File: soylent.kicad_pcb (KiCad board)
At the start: 2 copper layers, 33 x 42.2 mm, 31 parts, among them J1 DB9_Female, J2 Conn_01x04, J3 Conn_01x04, J4 Conn_02x03_Counter_Clockwise, Q1 BC847, Q2 BC847, U1 ATtiny202-SS, U2 MIC5504-3.3YM5, U3 LM2776, U4 MAX3188EEUT+T, U5 TLV6001DCK

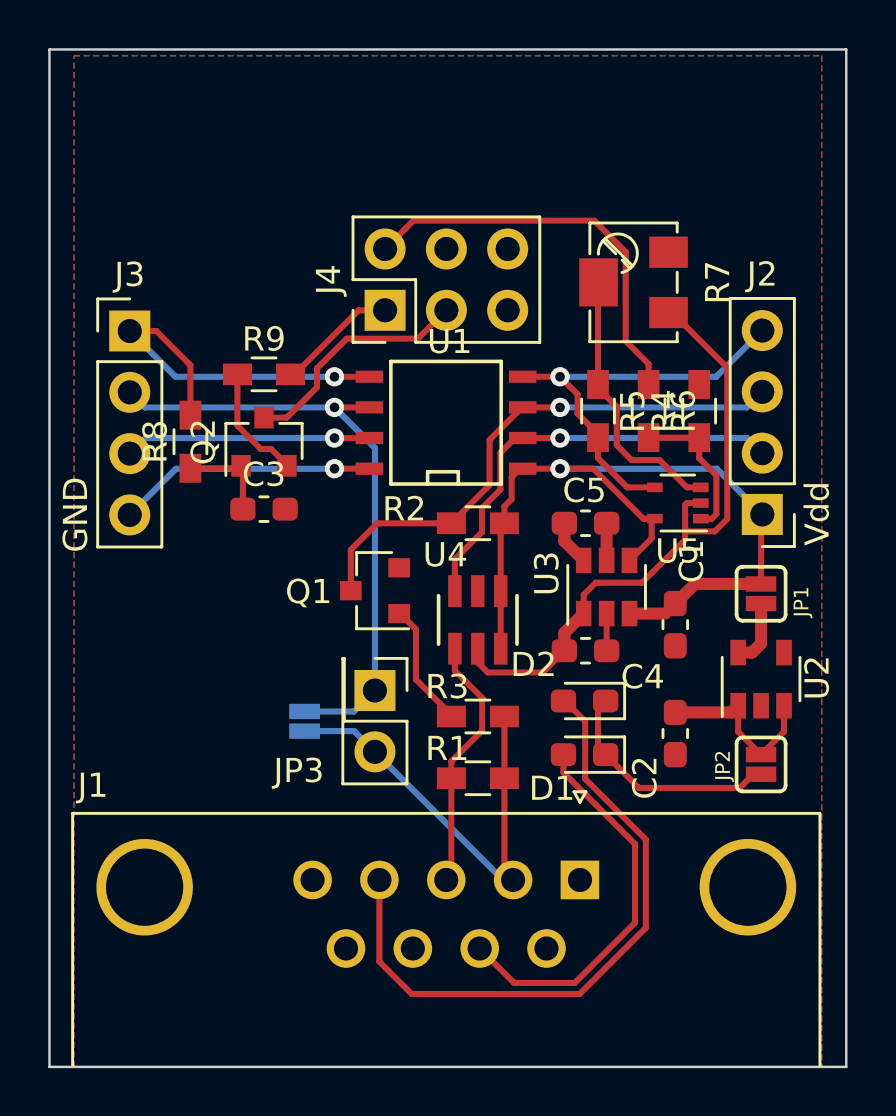
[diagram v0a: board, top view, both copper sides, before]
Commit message: Minor prettification
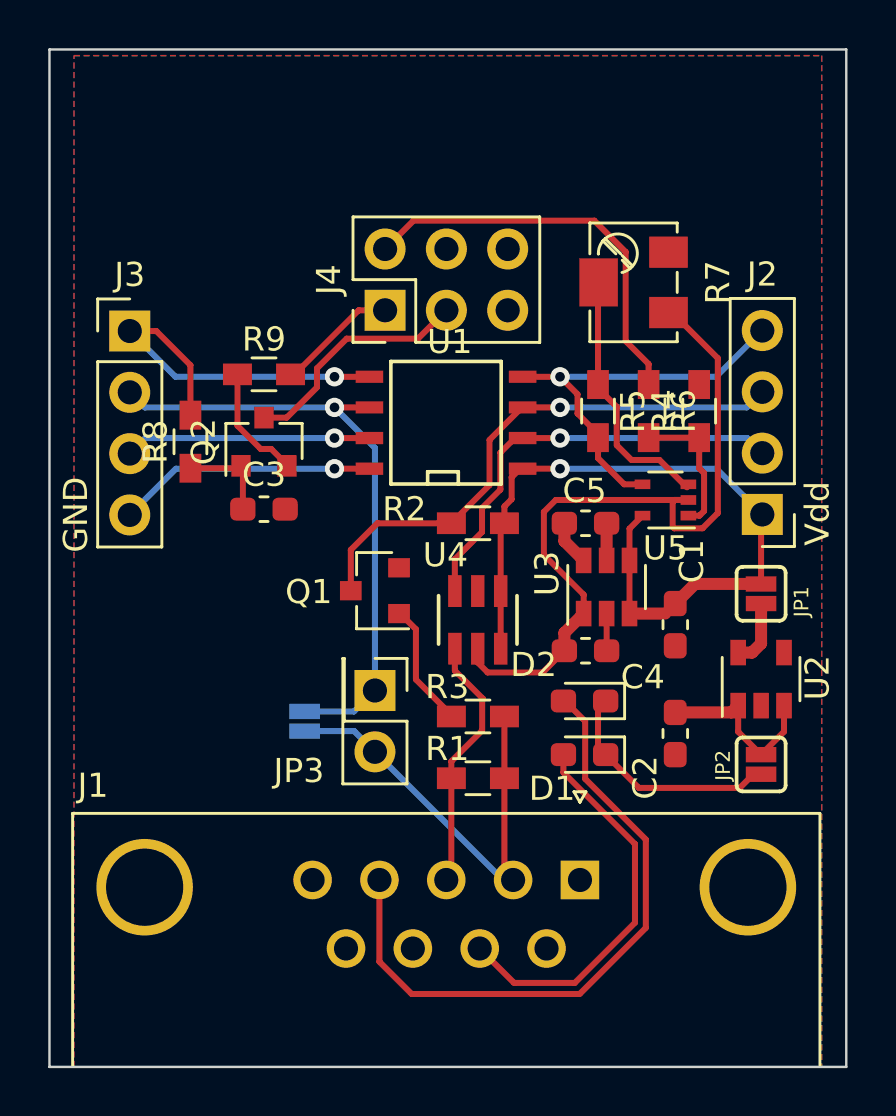
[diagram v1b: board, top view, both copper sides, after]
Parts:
- moved U5 0.53 mm to (248.3, 38.6)
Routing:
- net VEE: track 26.3 -> 30.8 mm
- net VDD: track 34.4 -> 31.8 mm
- net /WIN: track 17.7 -> 17.0 mm
- net Net-(R4-Pad1): track 6.29 -> 5.64 mm
- net Net-(R5-Pad1): track 11.3 -> 10.7 mm
